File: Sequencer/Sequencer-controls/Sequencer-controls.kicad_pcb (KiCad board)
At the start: 2 copper layers, 163.5 x 105.5 mm, 97 parts, among them SW1 SW_Push_DPDT, SW10 SW_SPDT, SW11 SW_SPDT, SW12 SW_SPDT, SW13 SW_SPDT, SW14 SW_SPDT, SW15 SW_SPDT, SW16 SW_SPDT, SW17 SW_SPDT, SW18 SW_SPDT, SW19 SW_SPDT, SW4 SW_SPDT, SW5 SW_SPDT, SW6 SW_SPDT, SW7 SW_SPDT, SW8 SW_SPDT, SW9 SW_SPDT

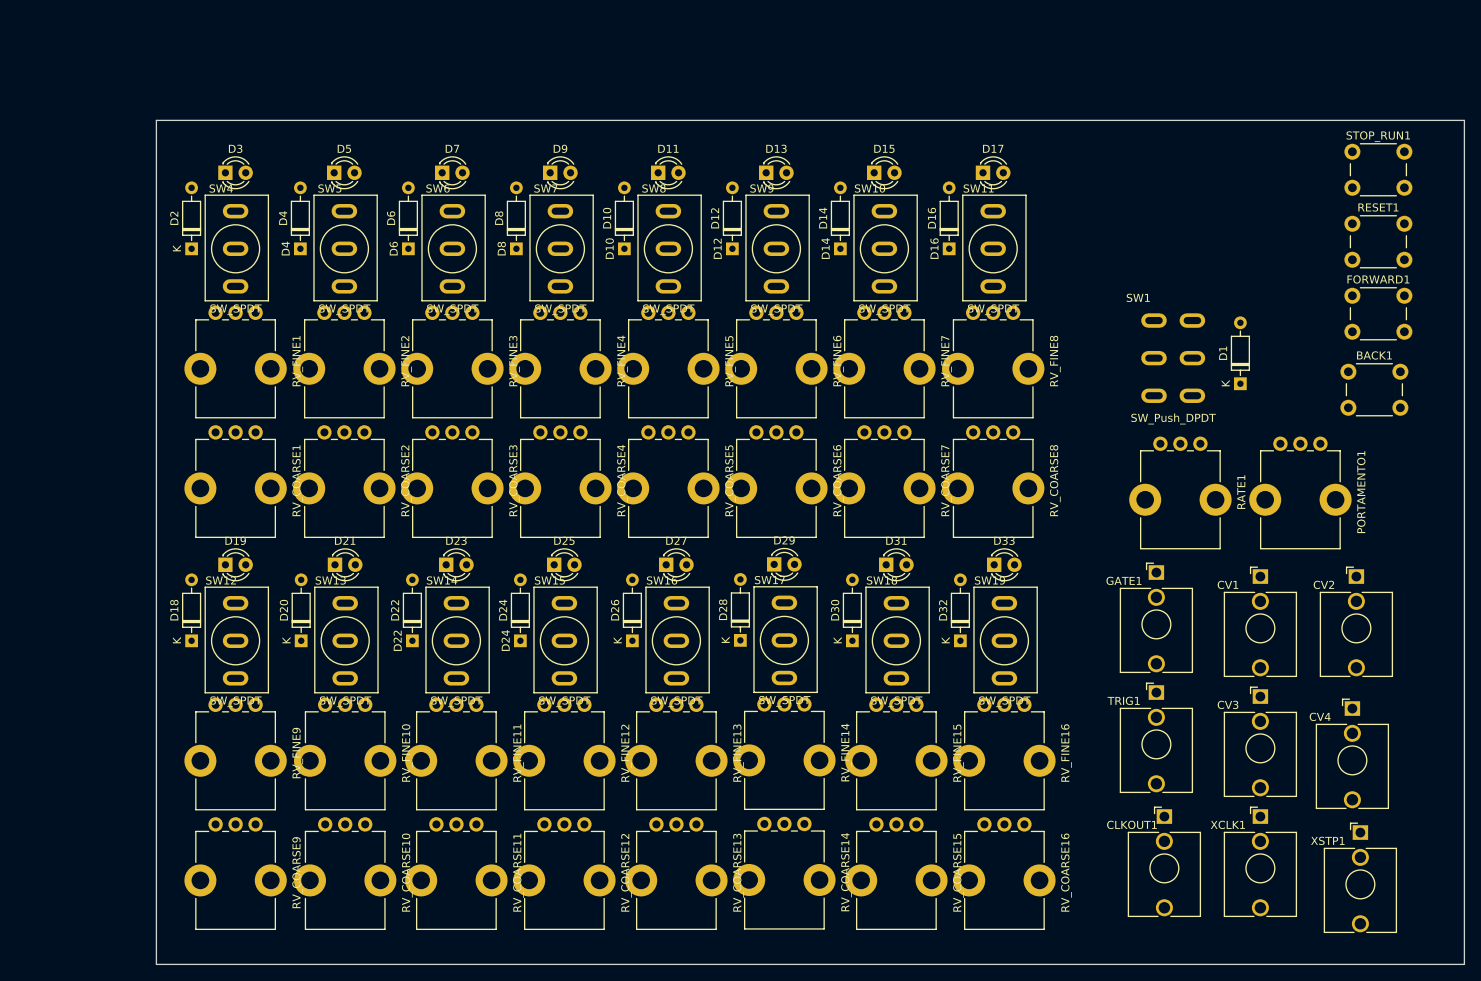
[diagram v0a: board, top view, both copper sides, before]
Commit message: just playing around
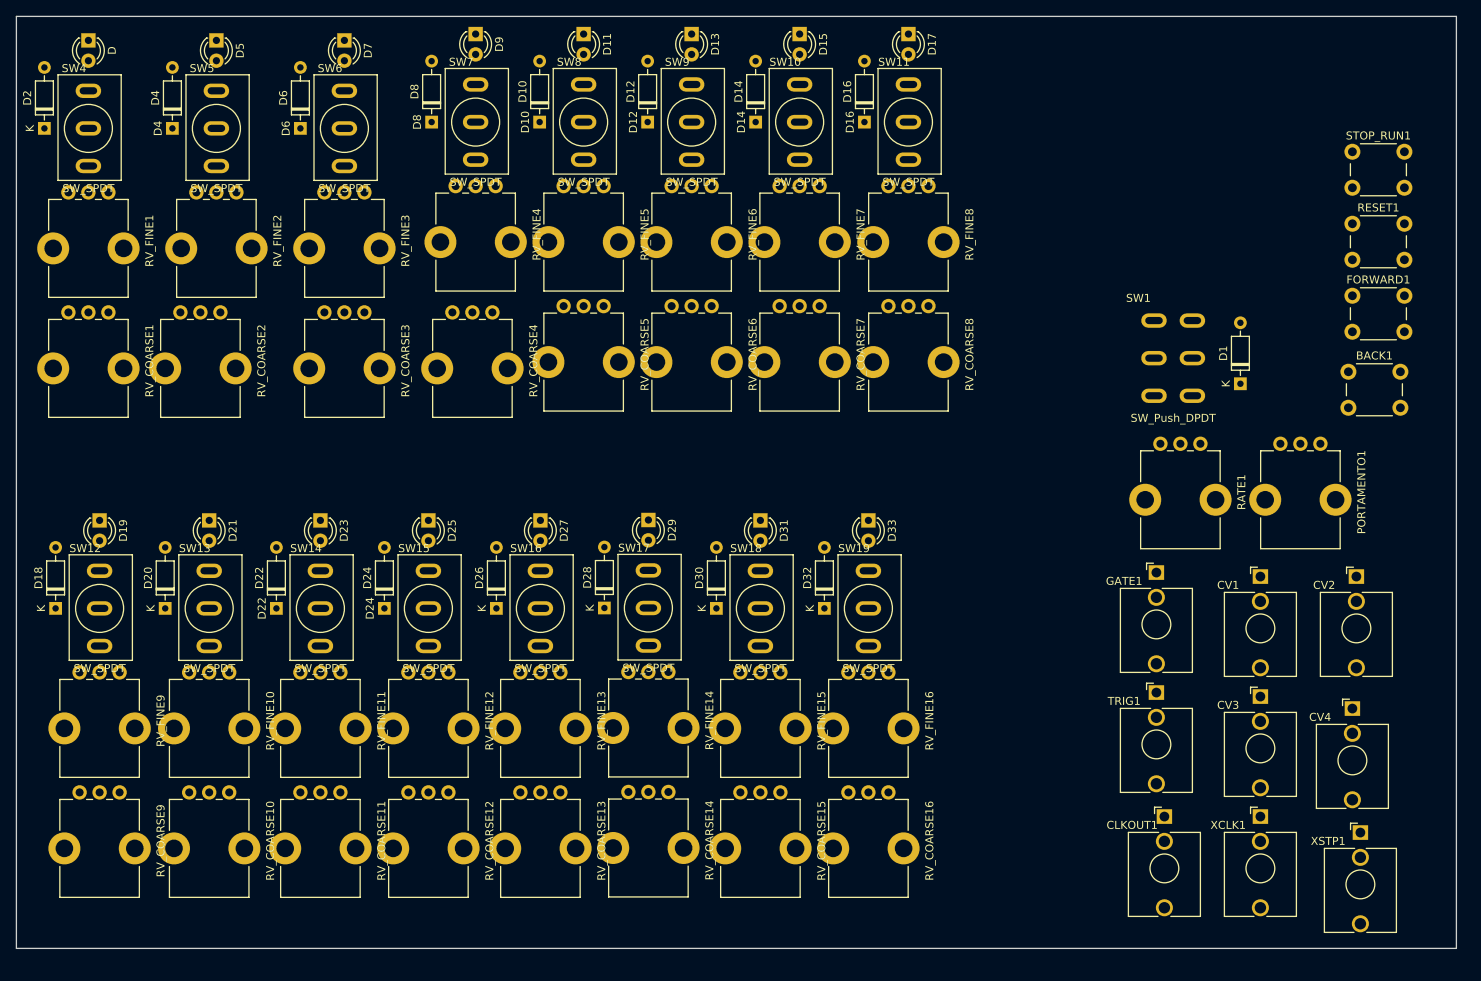
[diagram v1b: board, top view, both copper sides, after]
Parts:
- D  : renamed from D3
- moved D   23.8 mm to (9.00, 9.00), turned to -90 degrees
- moved D2 23.8 mm to (3.50, 20.0)
- moved RV_FINE1 23.8 mm to (9.00, 35.0)
- moved SW4 23.8 mm to (9.00, 20.0)
- moved RV_COARSE1 23.7 mm to (9.00, 50.0)
- moved RV_COARSE2 23.4 mm to (23.0, 50.0)
- moved D5 22.2 mm to (25.0, 9.00), turned to -90 degrees
- moved D4 22.0 mm to (19.5, 20.0)
- moved RV_FINE2 22.0 mm to (25.0, 35.0)
- moved SW5 22.0 mm to (25.0, 20.0)
- moved D7 20.6 mm to (41.0, 9.00), turned to -90 degrees
- moved D6 20.2 mm to (35.5, 20.0)
- moved RV_FINE3 20.2 mm to (41.0, 35.0)
- moved SW6 20.2 mm to (41.0, 20.0)
- moved RV_COARSE3 20.2 mm to (41.0, 50.0)
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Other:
- board size 163.5 x 105.5 mm -> 180 x 116.5 mm
